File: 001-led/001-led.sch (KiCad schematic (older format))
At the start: 3 parts

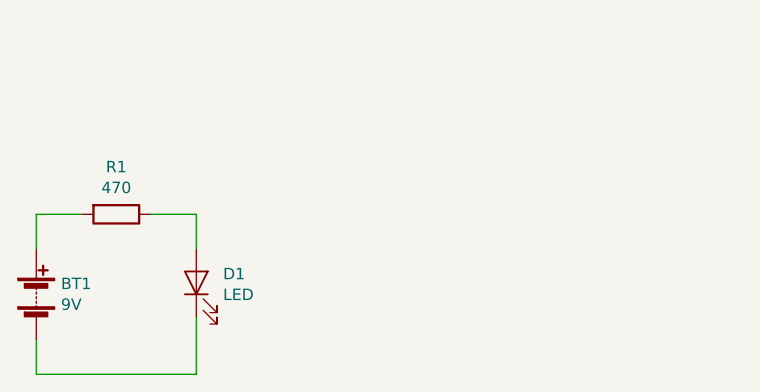
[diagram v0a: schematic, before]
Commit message: 001 again
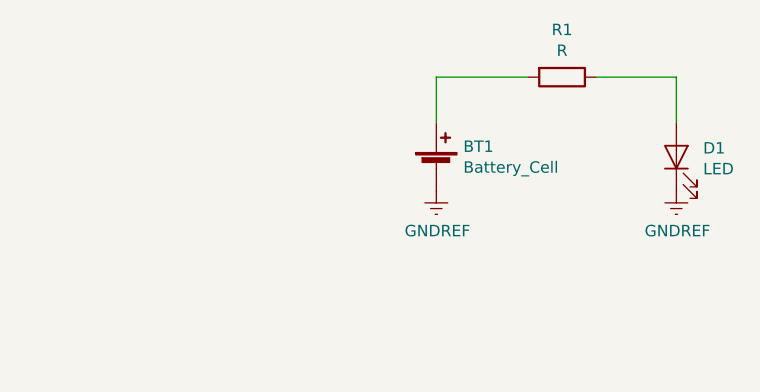
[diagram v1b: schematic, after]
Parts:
- removed BT1: 9V, Connector_PinHeader_2.54mm:PinHeader_1x02_P2.54mm_Vertical, symbol Device:Battery
- added BT1: Battery_Cell, Connector_PinHeader_2.54mm:PinHeader_1x02_P2.54mm_Vertical, symbol Device:Battery_Cell
- D1: footprint LED_SMD:LED_1206_3216Metric_Castellated -> LED_SMD:LED_0603_1608Metric
- R1: value 470 -> R; footprint Resistor_SMD:R_1206_3216Metric -> Resistor_SMD:R_0603_1608Metric
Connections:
- net at R1.2: now also BT1.1 (+)
- net GNDREF: now reaches D1.1 (K)
- net GNDREF: now also BT1.2 (-)
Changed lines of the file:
@@
 $Comp
 L Device:R R1
-U 1 1 5D9EEF0E
-P 3650 4150
-F 0 "R1" V 3443 4150 50  0000 C CNN
-F 1 "470" V 3534 4150 50  0000 C CNN
-F 2 "Resistor_SMD:R_1206_3216Metric" V 3580 4150 50  0001 C CNN
-F 3 "~" H 3650 4150 50  0001 C CNN
-	1    3650 4150
+U 1 1 5E2612B1
+P 5600 3550
+F 0 "R1" V 5393 3550 50  0000 C CNN
+F 1 "R" V 5484 3550 50  0000 C CNN
+F 2 "Resistor_SMD:R_0603_1608Metric" V 5530 3550 50  0001 C CNN
+F 3 "~" H 5600 3550 50  0001 C CNN
+	1    5600 3550
 	0    1    1    0
 $EndComp
 $Comp
 L Device:LED D1
-U 1 1 5D9EF8D8
-P 4000 4450
-F 0 "D1" V 4039 4333 50  0000 R CNN
-F 1 "LED" V 3948 4333 50  0000 R CNN
-F 2 "LED_SMD:LED_1206_3216Metric_Castellated" H 4000 4450 50  0001 C CNN
-F 3 "~" H 4000 4450 50  0001 C CNN
-	1    4000 4450
+U 1 1 5E261985
+P 6100 3900
+F 0 "D1" V 6139 3783 50  0000 R CNN
+F 1 "LED" V 6048 3783 50  0000 R CNN
+F 2 "LED_SMD:LED_0603_1608Metric" H 6100 3900 50  0001 C CNN
+F 3 "~" H 6100 3900 50  0001 C CNN
+	1    6100 3900
 	0    -1   -1   0
 $EndComp
 $Comp
-L Device:Battery BT1
-U 1 1 5D9F0396
-P 3300 4500
-F 0 "BT1" H 3408 4546 50  0000 L CNN
-F 1 "9V" H 3408 4455 50  0000 L CNN
-F 2 "Connector_PinHeader_2.54mm:PinHeader_1x02_P2.54mm_Vertical" V 3300 4560 50  0001 C CNN
-F 3 "~" V 3300 4560 50  0001 C CNN
-	1    3300 4500
+L Device:Battery_Cell BT1
+U 1 1 5E2624A7
+P 5050 3950
+F 0 "BT1" H 5168 4046 50  0000 L CNN
+F 1 "Battery_Cell" H 5168 3955 50  0000 L CNN
+F 2 "Connector_PinHeader_2.54mm:PinHeader_1x02_P2.54mm_Vertical" V 5050 4010 50  0001 C CNN
+F 3 "~" V 5050 4010 50  0001 C CNN
+	1    5050 3950
 	1    0    0    -1
 $EndComp
 Wire Wire Line
-	3300 4300 3300 4150
+	5050 3750 5050 3550
 Wire Wire Line
-	3300 4150 3500 4150
+	5050 3550 5450 3550
 Wire Wire Line
-	3800 4150 4000 4150
+	5750 3550 6100 3550
 Wire Wire Line
-	4000 4150 4000 4300
-Wire Wire Line
-	4000 4600 4000 4850
-Wire Wire Line
-	4000 4850 3300 4850
-Wire Wire Line
-	3300 4850 3300 4700
+	6100 3550 6100 3750
+$Comp
+L power:GNDREF #PWR?
+U 1 1 5E262E93
+P 5050 4050
+F 0 "#PWR?" H 5050 3800 50  0001 C CNN
+F 1 "GNDREF" H 5055 3877 50  0000 C CNN
+F 2 "" H 5050 4050 50  0001 C CNN
+F 3 "" H 5050 4050 50  0001 C CNN
+	1    5050 4050
+	1    0    0    -1
+$EndComp
+$Comp
+L power:GNDREF #PWR?
+U 1 1 5E26336D
+P 6100 4050
+F 0 "#PWR?" H 6100 3800 50  0001 C CNN
+F 1 "GNDREF" H 6105 3877 50  0000 C CNN
+F 2 "" H 6100 4050 50  0001 C CNN
+F 3 "" H 6100 4050 50  0001 C CNN
+	1    6100 4050
+	1    0    0    -1
+$EndComp
 $EndSCHEMATC
